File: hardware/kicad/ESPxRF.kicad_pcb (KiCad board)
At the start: 4 copper layers, 67.6 x 28.7 mm, 36 parts, among them J1 USB_C_Receptacle_USB2.0, J2 ANT, U1 USBLC6-2SC6, U2 NCP115ASN330T2G, U3 ESP32-S3, U4 NRF24L01, Y1 Crystal_GND24_Small

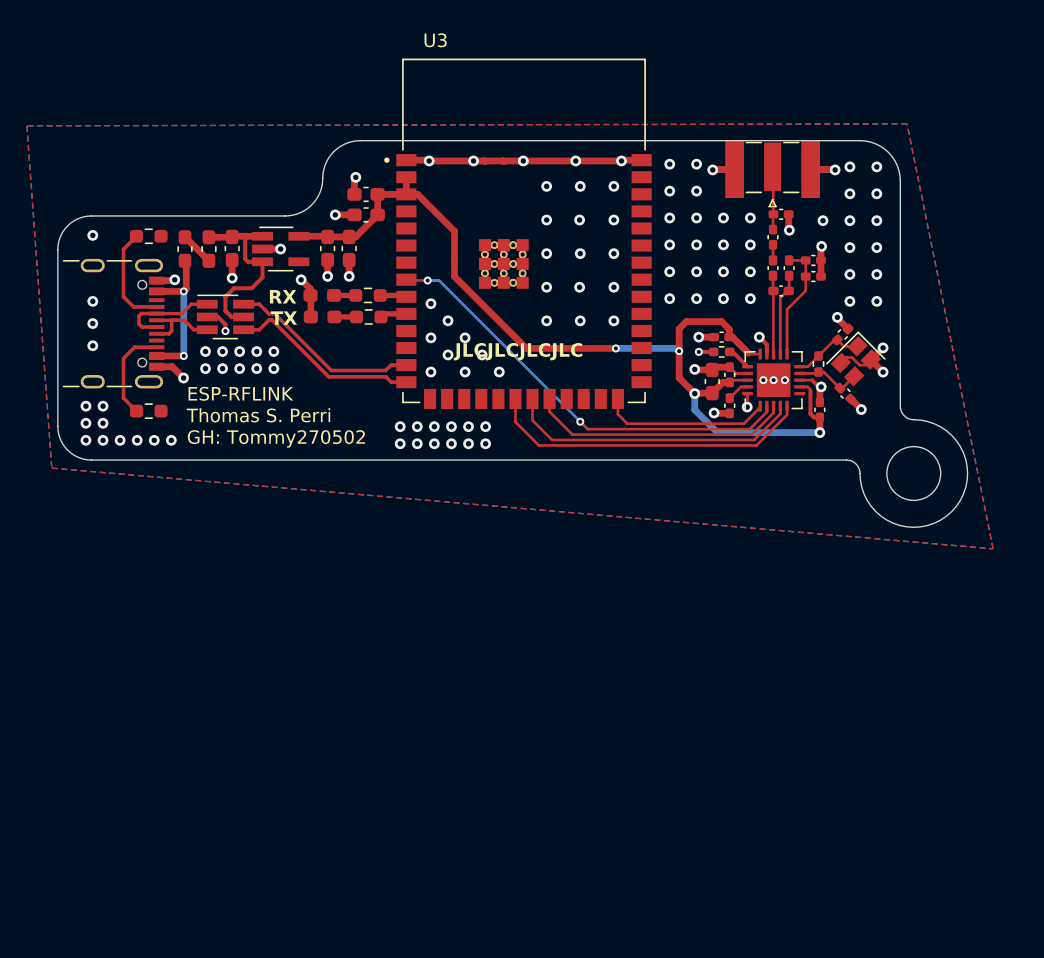
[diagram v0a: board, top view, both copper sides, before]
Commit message: V2
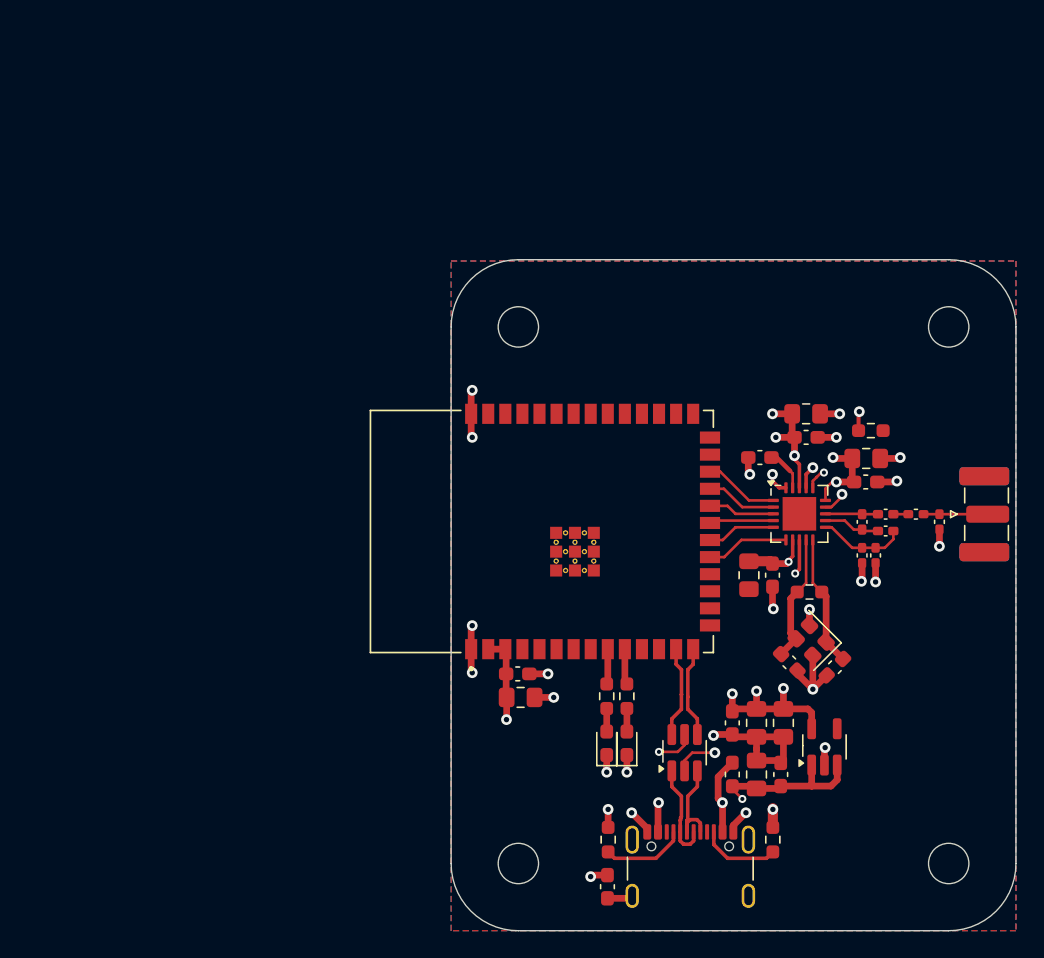
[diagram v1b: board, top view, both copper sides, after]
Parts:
- removed L4: 2n7, Inductor_SMD:L_0402_1005Metric_Pad0.77x0.64mm_HandSolder
- added C18: 4p7, Capacitor_SMD:C_0402_1005Metric_Pad0.74x0.62mm_HandSolder, F.Cu at (146.1, 90.1)
- added C19: 100n, Capacitor_SMD:C_0603_1608Metric_Pad1.08x0.95mm_HandSolder, F.Cu at (146.4, 84.6)
- added C20: 1p5, Capacitor_SMD:C_0402_1005Metric_Pad0.74x0.62mm_HandSolder, F.Cu at (150.1, 87.0)
- added C21: 1p, Capacitor_SMD:C_0402_1005Metric_Pad0.74x0.62mm_HandSolder, F.Cu at (151.9, 87.6)
- added C4: 10u, Capacitor_SMD:C_0805_2012Metric_Pad1.18x1.45mm_HandSolder, F.Cu at (120.7, 100.7)
- C1, C5, C8: value 10u -> 100n
- C10, C13: value 100n -> 10u; footprint Capacitor_SMD:C_0402_1005Metric_Pad0.74x0.62mm_HandSolder -> Capacitor_SMD:C_0805_2012Metric_Pad1.18x1.45mm_HandSolder
- C11: value 22p -> 10u; footprint Capacitor_SMD:C_0402_1005Metric_Pad0.74x0.62mm_HandSolder -> Capacitor_SMD:C_0805_2012Metric_Pad1.18x1.45mm_HandSolder
- C12: value 2n2 -> 22p; footprint Capacitor_SMD:C_0402_1005Metric_Pad0.74x0.62mm_HandSolder -> Capacitor_SMD:C_0603_1608Metric_Pad1.08x0.95mm_HandSolder
- C14: value 4p7 -> 100n; footprint Capacitor_SMD:C_0402_1005Metric_Pad0.74x0.62mm_HandSolder -> Capacitor_SMD:C_0603_1608Metric_Pad1.08x0.95mm_HandSolder
- C15: value 100n -> 22p; footprint Capacitor_SMD:C_0402_1005Metric_Pad0.74x0.62mm_HandSolder -> Capacitor_SMD:C_0603_1608Metric_Pad1.08x0.95mm_HandSolder
- C16: value 1p5 -> 2n2
- C17: value 1p -> 100n; footprint Capacitor_SMD:C_0402_1005Metric_Pad0.74x0.62mm_HandSolder -> Capacitor_SMD:C_0603_1608Metric_Pad1.08x0.95mm_HandSolder
- C2: footprint Capacitor_SMD:C_0603_1608Metric_Pad1.08x0.95mm_HandSolder -> Capacitor_SMD:C_0805_2012Metric_Pad1.18x1.45mm_HandSolder
- C6: value 100n -> 10u; footprint Capacitor_SMD:C_0603_1608Metric_Pad1.08x0.95mm_HandSolder -> Capacitor_SMD:C_0805_2012Metric_Pad1.18x1.45mm_HandSolder
- C7: value 33n -> 10u; footprint Capacitor_SMD:C_0402_1005Metric_Pad0.74x0.62mm_HandSolder -> Capacitor_SMD:C_0805_2012Metric_Pad1.18x1.45mm_HandSolder
- C9: value 22p -> 33n; footprint Capacitor_SMD:C_0402_1005Metric_Pad0.74x0.62mm_HandSolder -> Capacitor_SMD:C_0603_1608Metric_Pad1.08x0.95mm_HandSolder
- J2: footprint Connector_Coaxial:SMA_Samtec_SMA-J-P-X-ST-EM1_EdgeMount -> Connector_Coaxial:SMA_Samtec_SMA-J-P-H-ST-EM1_EdgeMount
- L1: value 2u2 -> 8n2; footprint Inductor_SMD:L_0603_1608Metric_Pad1.05x0.95mm_HandSolder -> Inductor_SMD:L_0402_1005Metric_Pad0.77x0.64mm_HandSolder
- L2: value 8n2 -> 3n9
- L3: value 3n9 -> 2n7
- R1: value 5k1 -> 1k3
- R3: value 1k3 -> 5k1
- R5, R6: footprint Resistor_SMD:R_0402_1005Metric_Pad0.72x0.64mm_HandSolder -> Resistor_SMD:R_0603_1608Metric_Pad0.98x0.95mm_HandSolder
- U1: value USBLC6-2SC6 -> ESP32-S3; footprint Package_TO_SOT_SMD:SOT-23-6_Handsoldering -> ESP32-S3-WROOM:XCVR_ESP32S3WROOM1N8R8
- U2: value NCP115ASN330T2G -> USBLC6-2SC6; footprint Package_TO_SOT_SMD:SOT-23-5_HandSoldering -> Package_TO_SOT_SMD:SOT-23-6_Handsoldering
- U3: value ESP32-S3 -> NCP115ASN330T2G; footprint ESP32:XCVR_ESP32S3WROOM1N8R8 -> Package_TO_SOT_SMD:SOT-23-5_HandSoldering
- moved R2 64.5 mm to (139.5, 111.2), turned to 90 degrees
- moved J1 60.0 mm to (133.3, 114.3), turned to 0 degrees
- moved F1 56.4 mm to (136.5, 106.4), turned to -90 degrees
- moved C1 55.1 mm to (127.2, 114.7), turned to 90 degrees
- moved L1 52.6 mm to (146.1, 87.6), turned to -90 degrees
- moved C3 50.6 mm to (140.1, 106.4), turned to 90 degrees
- moved C2 50.5 mm to (138.3, 106.4), turned to 90 degrees
- moved C6 48.9 mm to (138.3, 102.5), turned to -90 degrees
- moved U2 48.0 mm to (132.9, 104.8), turned to 90 degrees
- moved U3 44.4 mm to (143.3, 104.3), turned to 90 degrees
- moved R3 44.2 mm to (127.2, 111.2), turned to 90 degrees
- moved R1 40.1 mm to (127.1, 100.6), turned to -90 degrees
- moved D1 39.5 mm to (127.1, 104.1), turned to 90 degrees
- moved D2 38.9 mm to (128.6, 104.1), turned to 90 degrees
- moved C5 35.9 mm to (120.5, 98.9), turned to 0 degrees
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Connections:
- C1 pad 1: +5V -> Net-(J1-SHIELD)
- C11 pad 1: XC2 -> +3V3
- C12 pad 1: VDD_PA -> XC1
- C14 pad 1: VDD_PA -> +3V3
- C15 pad 1: +3V3 -> XC2
- C16 pad 1: Net-(C16-Pad1) -> VDD_PA
- C16 pad 2: Net-(J2-In) -> GND
- C17 pad 1: Net-(J2-In) -> +3V3
- C2 pad 1: +3V3 -> +5V
- C3 pad 1: +3V3 -> +5V
- C7 pad 1: Net-(U4-DVDD) -> +3V3
- C9 pad 1: XC1 -> Net-(U4-DVDD)
- F1 pad 2: Net-(F1-Pad2) -> +5V
- J1 pad S1: unconnected-(J1-SHIELD-PadS1) -> Net-(J1-SHIELD)
- L1 pad 1: Net-(F1-Pad2) -> ANT2
- L1 pad 2: +5V -> ANT1
- L2 pad 2: ANT1 -> Net-(C20-Pad1)
- L3 pad 1: ANT2 -> ANT1
- L3 pad 2: Net-(C16-Pad1) -> VDD_PA
- R1 pad 1: Net-(J1-CC2) -> Net-(U1-IO16)
- R1 pad 2: GND -> Net-(D1-A)
- R2 pad 1: Net-(J1-CC1) -> Net-(J1-CC2)
- R3 pad 1: Net-(U3-IO16) -> Net-(J1-CC1)
- R3 pad 2: Net-(D1-A) -> GND
- R4 pad 1: Net-(U3-IO17) -> Net-(U1-IO17)
- U1 pad 1: USBCON_D- -> GND
- U1 pad 2: GND -> +3V3
- U1 pad 3: USBCON_D+ -> +3V3
- U1 pad 4: USB_D+ -> unconnected-(U1-IO4-Pad4)
- U1 pad 5: +5V -> unconnected-(U1-IO5-Pad5)
- U1 pad 6: USB_D- -> unconnected-(U1-IO6-Pad6)
- U2 pad 1: +5V -> USBCON_D-
- U2 pad 3: +5V -> USBCON_D+
- U2 pad 4: (no net) -> USB_D+
- U2 pad 5: +3V3 -> +5V
- U3 pad 1: GND -> +5V
- U3 pad 2: +3V3 -> GND
- U3 pad 3: +3V3 -> +5V
- U3 pad 4: unconnected-(U3-IO4-Pad4) -> (no net)
- U3 pad 5: unconnected-(U3-IO5-Pad5) -> +3V3
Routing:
- net +3V3: track 71.8 -> 37.9 mm, vias 4 -> 10
- net CSN: track 32.4 -> 5.27 mm, vias 2 -> 0
- net GND: track 84.0 -> 63.6 mm, vias 126 -> 31
- net MISO: track 24.2 -> 5.10 mm
- net Net-(J1-SHIELD): track 0.00 -> 18.9 mm
- net MOSI: track 22.0 -> 4.78 mm
- net SCK: track 19.5 -> 4.96 mm
- net +5V: track 14.2 -> 22.6 mm, vias 0 -> 2
- net Net-(U4-IREF): track 1.78 -> 9.41 mm, vias 0 -> 2
- net USB_D+: track 14.3 -> 6.81 mm
- net USB_D-: track 14.3 -> 6.81 mm
- net CE: track 12.6 -> 5.59 mm
- net IRQ: track 0.00 -> 6.18 mm
- net XC2: track 4.97 -> 9.60 mm
- net XC1: track 5.33 -> 9.79 mm
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- added copper zone on In2.Cu, net +3V3
- removed copper zone on In2.Cu, net GND
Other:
- board size 67.6 x 28.7 mm -> 42 x 49.9 mm
- board text removed: "ESP-RFLINK Thomas S. Perri GH: Tommy270502"
- board text removed: "JLCJLCJLCJLC"
- board text removed: "RX"
- board text removed: "TX"
